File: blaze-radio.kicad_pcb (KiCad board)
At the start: 4 copper layers, 16 x 16 mm, 44 parts, among them J1 Conn_02x08_Castelated, J2 TagConnect_TC2030, U1 EFR32xG23xxxxF512xM48, U2 TSS-13HLN+, Y1 32.768KHz, Y2 38.400MHz

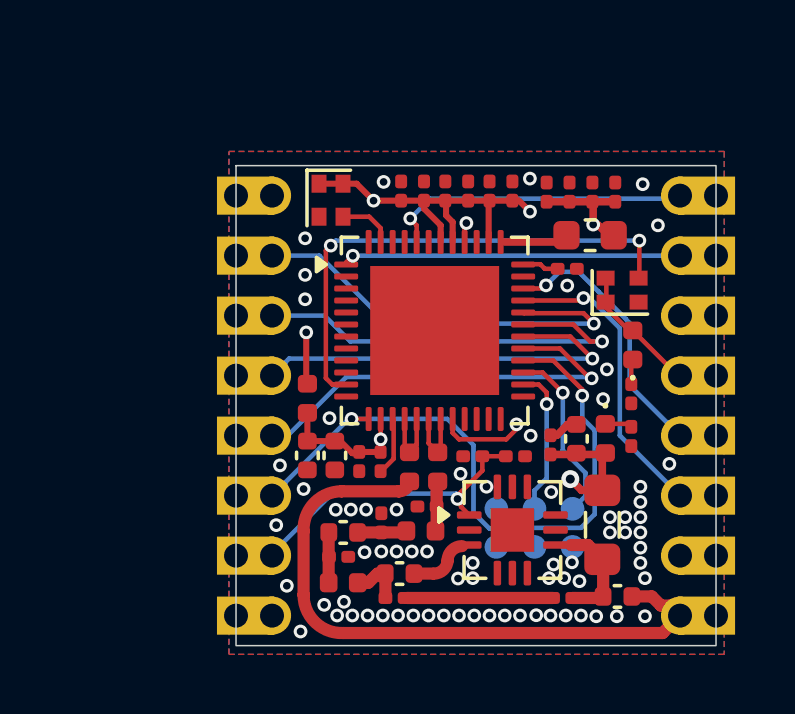
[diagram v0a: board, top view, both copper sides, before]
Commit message: Routing updates
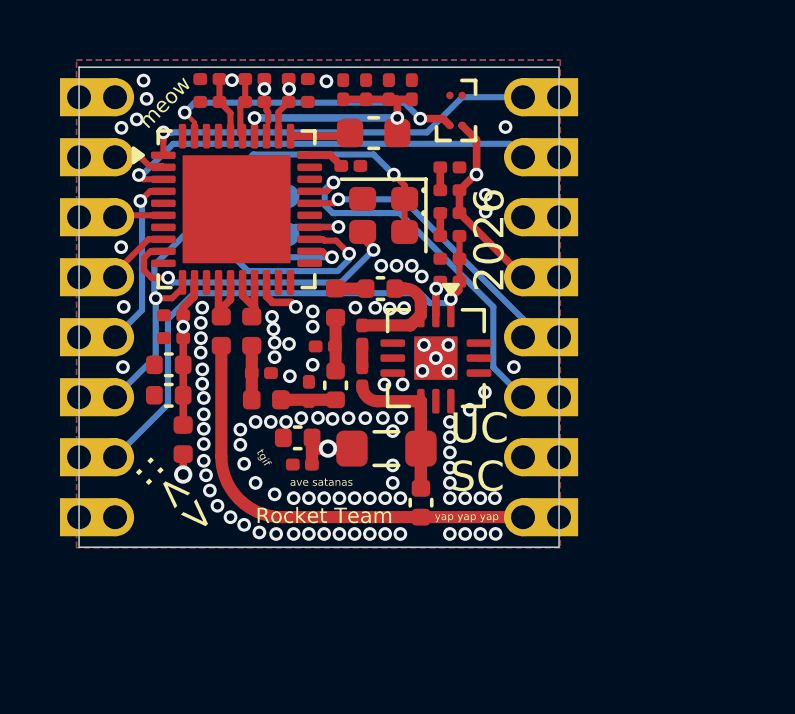
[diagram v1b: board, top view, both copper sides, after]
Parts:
- removed Y1: 32.768KHz, Oscillator:Oscillator_SMD_Abracon_ASCO-4Pin_1.6x1.2mm
- added Y3: 32.768KHz, Avionics_Feet:OSC_SIT1532AI-J4-DCC-32.768D, F.Cu at (105.6, 59.1)
- D1, D2: footprint LED_SMD:LED_0402_1005Metric -> LED_SMD:LED_0201_0603Metric
- U1: value EFR32xG23xxxxF512xM48 -> EFR32FG23A010F256GM40; footprint Package_DFN_QFN:QFN-48-1EP_6x6mm_P0.4mm_EP4.3x4.3mm -> Package_DFN_QFN:QFN-40-1EP_5x5mm_P0.4mm_EP3.6x3.6mm
- Y2: value 38.400MHz -> 39MHz; footprint Oscillator:Oscillator_SMD_Abracon_ASCO-4Pin_1.6x1.2mm -> Crystal:Crystal_SMD_2016-4Pin_2.0x1.6mm
- moved J2 14.1 mm to (98.7, 62.6), turned to 0 degrees
- moved R3 9.95 mm to (102.5, 68.0), turned to -90 degrees
- moved R2 9.67 mm to (105.4, 61.0), turned to 0 degrees
- moved C23 9.52 mm to (103.1, 65.0)
- moved L7 9.32 mm to (101.6, 65.5), turned to 90 degrees
- moved C20 9.29 mm to (100.3, 70.0), turned to 180 degrees
- moved D1 9.13 mm to (105.4, 62.5), turned to 0 degrees
- moved R1 9.01 mm to (105.4, 63.3), turned to 0 degrees
- moved C19 8.83 mm to (102.5, 66.6), turned to -90 degrees
- moved Y2 8.33 mm to (103.2, 62.6), turned to 180 degrees
- moved C22 8.30 mm to (100.5, 70.9), turned to 180 degrees
- moved C4 8.06 mm to (97.4, 58.0), turned to 180 degrees
- moved C13 8.03 mm to (96.2, 66.7), turned to 180 degrees
- moved C18 7.99 mm to (102.1, 60.9)
- moved D2 7.99 mm to (105.4, 61.7), turned to 0 degrees
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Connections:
- C19 pad 1: Net-(C19-Pad1) -> Net-(U2-IN)
- C23 pad 1: Net-(C19-Pad1) -> Net-(C23-Pad1)
- D1 pad 2: VDD -> +3V3
- J1 pad 15: /PC00 -> /PC02
- J1 pad 16: /PD04 -> /PC00
- L7 pad 2: Net-(C19-Pad1) -> Net-(C23-Pad1)
- R1 pad 2: GND -> /PA_nEN
- U1 pad 11: Net-(U1-HFXTAL_I) -> /nRST
- U1 pad 12: unconnected-(U1-HFXTAL_O-Pad12) -> VDDA
- U1 pad 13: /nRST -> GND
- U1 pad 14: VDDA -> /Transceiver/IN
- U1 pad 15: GND -> /Transceiver/IN
- U1 pad 16: /Transceiver/IN -> /Transceiver/OUT
- U1 pad 17: /Transceiver/IN -> /Transceiver/OUT
- U1 pad 18: /Transceiver/OUT -> VDDA
- U1 pad 19: /Transceiver/OUT -> unconnected-(U1-PB01-Pad19)
- U1 pad 2: unconnected-(U1-PC01-Pad2) -> /MISO
- U1 pad 20: VDDA -> unconnected-(U1-PB00-Pad20)
- U1 pad 22: unconnected-(U1-PB02-Pad22) -> /Transceiver/SWCLK
- U1 pad 23: unconnected-(U1-PB01-Pad23) -> /Transceiver/SWDIO
- U1 pad 24: unconnected-(U1-PB00-Pad24) -> /Transceiver/SWO
- U1 pad 26: /Transceiver/SWCLK -> /UART_RX
- U1 pad 27: /Transceiver/SWDIO -> /UART_TX
- U1 pad 28: /Transceiver/SWO -> unconnected-(U1-PA07-Pad28)
- U1 pad 29: /CS -> unconnected-(U1-PA08-Pad29)
- U1 pad 3: unconnected-(U1-PC02-Pad3) -> /PC02
- U1 pad 30: /SCK -> Net-(U1-DECOUPLE)
- U1 pad 31: /MOSI -> Net-(U1-VREGSW)
- U1 pad 32: /MISO -> +3V3
- U1 pad 33: /UART_TX -> GND
- U1 pad 34: /UART_RX -> VDCDC
- U1 pad 35: unconnected-(U1-PA10-Pad35) -> +3V3
- U1 pad 36: Net-(U1-DECOUPLE) -> +3V3
- U1 pad 37: Net-(U1-VREGSW) -> unconnected-(U1-PD03-Pad37)
- U1 pad 38: +3V3 -> unconnected-(U1-PD02-Pad38)
- U1 pad 39: GND -> Net-(U1-PD01_LFXI)
- U1 pad 4: unconnected-(U1-PC03-Pad4) -> /CS
- U1 pad 40: VDCDC -> unconnected-(U1-PD00_LFXO-Pad40)
- U1 pad 41: +3V3 -> GND
- U1 pad 6: unconnected-(U1-PC05-Pad6) -> /MOSI
- U1 pad 8: unconnected-(U1-PC07-Pad8) -> /SCK
- U1 pad 9: unconnected-(U1-PC08-Pad9) -> Net-(U1-HFXTAL_I)
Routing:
- net +3V3: track 16.2 -> 31.9 mm, vias 3 -> 4
- net /PC02: track 0.00 -> 14.3 mm, vias 0 -> 1
- net /MOSI: track 14.7 -> 1.55 mm, vias 1 -> 0
- net /MISO: track 14.6 -> 1.75 mm, vias 1 -> 0
- net /SCK: track 14.0 -> 2.22 mm, vias 1 -> 0
- net /PD04: track 10.6 -> 0.00 mm, vias 1 -> 0
- net /CS: track 14.4 -> 5.84 mm
- net Net-(U1-PD01_LFXI): track 1.88 -> 10.2 mm, vias 0 -> 2
- net /Transceiver/SWO: track 10.5 -> 2.76 mm
- net /PA_nEN: track 10.5 -> 18.1 mm
- net Net-(U1-HFXTAL_I): track 16.6 -> 10.2 mm
- net /ANTENNA: track 18.0 -> 11.7 mm
- net VDCDC: track 17.6 -> 23.2 mm
- net Net-(C19-Pad2): track 4.87 -> 0.76 mm
- net Net-(U2-OUT): track 3.61 -> 7.27 mm
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- added copper zone on In2.Cu, net GND
- removed copper zone on In2.Cu, net +3V3
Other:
- board text added: "2026"
- board text added: "433MHz 50Ω"
- board text added: "::<>"
- board text added: "Rocket Team"
- board text added: "UC SC"
- board text added: "ave satanas"
- board text added: "meow"
- board text added: "tgif"
- board text added: "yap yap yap"
